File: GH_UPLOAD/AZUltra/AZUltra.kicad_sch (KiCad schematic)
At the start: 23 parts, among them Q1 SSM3J338R,LF, SW1 SW_DIP_x03, U1 TPS613222ADBV, U2 CH32V005

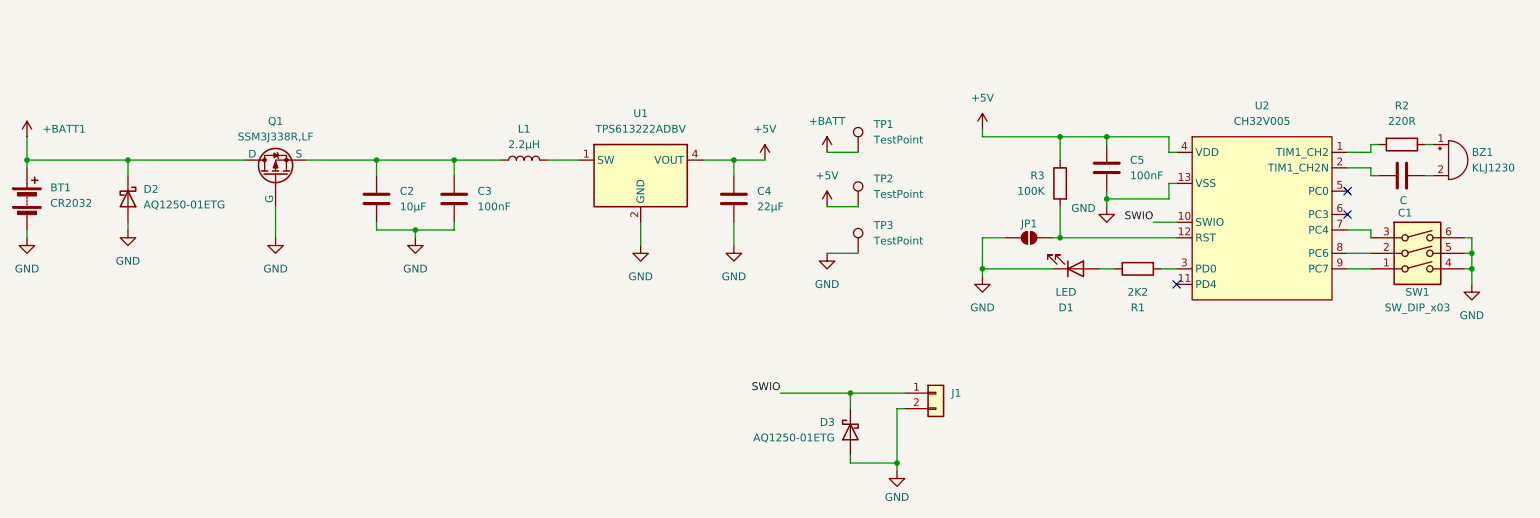
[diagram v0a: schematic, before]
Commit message: Update schematic
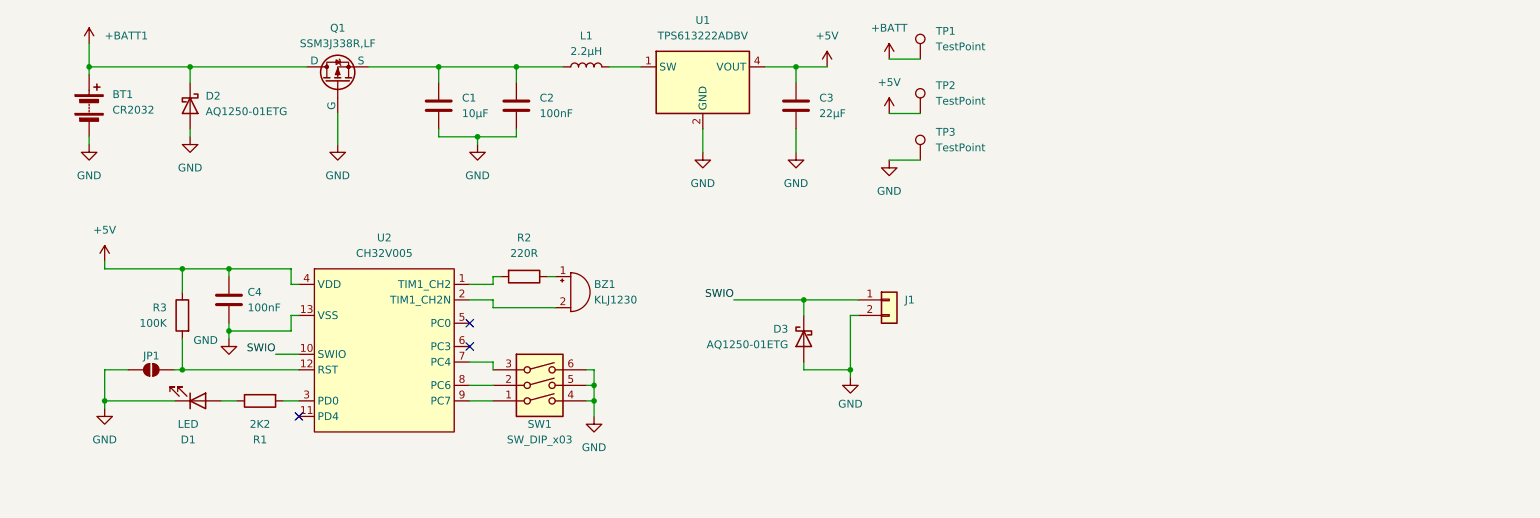
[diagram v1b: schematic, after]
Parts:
- removed C1: C, symbol Device:C
- renumbered C2 to C1, C3 to C2, C4 to C3, C5 to C4
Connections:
- net at U2.2 (PA2): now also BZ1.2 (-)
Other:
- company: (none) -> Adam Zembrzuski
- title: (none) -> AZUltra
- moved on the sheet: BT1, BZ1, C1, C2, C3, C4, D1, D2, D3, J1, JP1, L1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
